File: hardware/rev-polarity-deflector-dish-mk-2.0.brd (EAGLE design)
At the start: 22.9 x 17.8 mm, 13 parts, among them U1_ ROTARY_ENCODER_SWITCH, U2 Tiny85

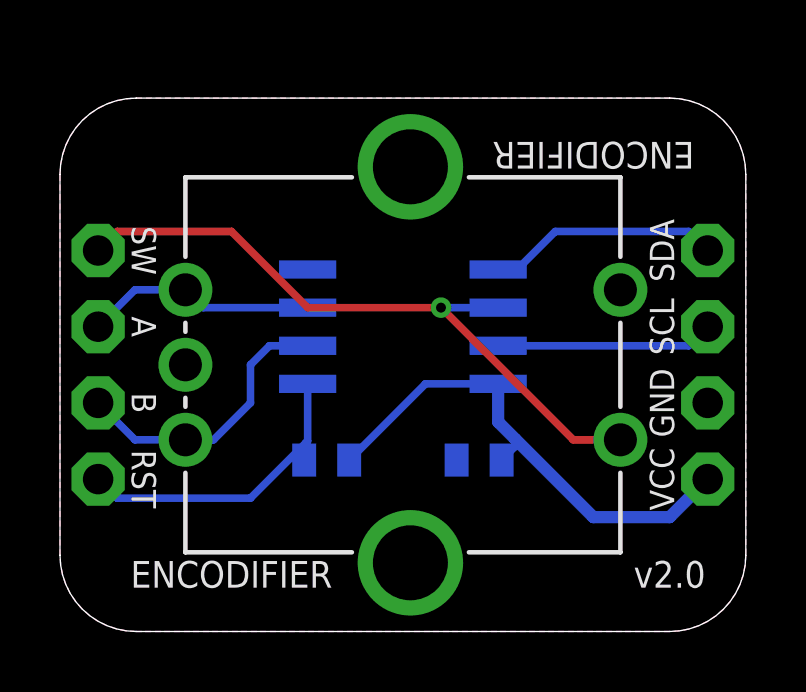
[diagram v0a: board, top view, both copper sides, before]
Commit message: have some boards, dawg
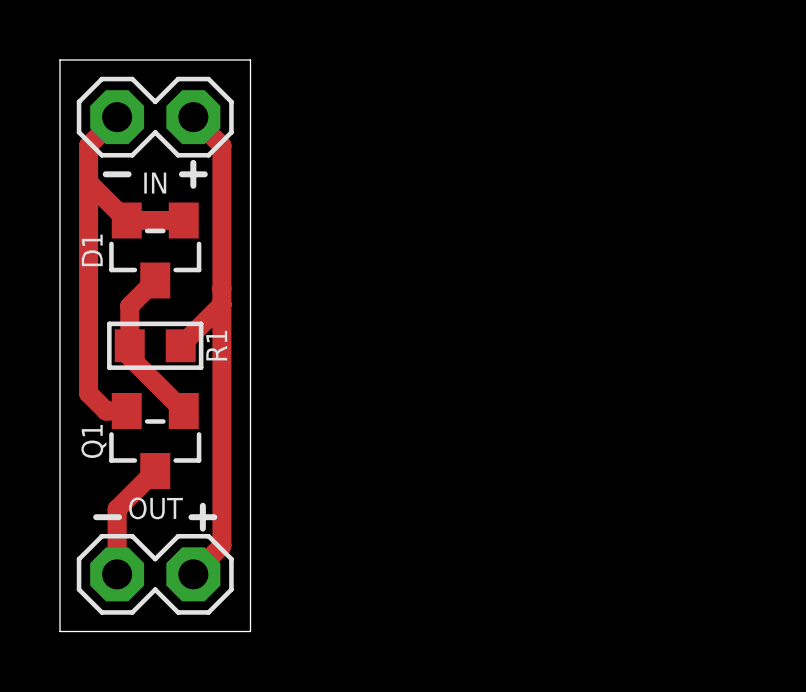
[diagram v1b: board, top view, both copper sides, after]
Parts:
- removed A, B, GND, RST, SCL, SDA, SW, VCC: M01PTH-1MM, a_parts:1X01-1MM-NS
- removed C1: 100n, a_parts:C0603-TIGHTER
- removed U1_: ROTARY_ENCODER_SWITCH, a_parts:ROTARY_ENCODER_SWITCH
- removed U2: Tiny85, a_parts:SO08-EIAJ
- added D1: 1N4740, a_parts:SOT23
- added IN, OUT: M02PTH-CENTERED, a_parts:1X02-CENTER
- added Q1: 2N7000, a_parts:SOT23
- R1: value 10k -> 100K; device a_parts:R0603-TIGHTER -> a_parts:R0603
- moved R1 6.87 mm to (3.17, 9.53), flipped to the top
- moved FRAME1 0.90 mm to (0.64, 0.64)
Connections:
- removed net A: A.1, U1_.A, U2.3
- removed net B: B.1, U1_.B, U2.2
- removed net GND: C1.2, GND.1, U1_.C, U1_.SW2, U2.4
- removed net MOSI/SDA: SDA.1, U2.5
- removed net RST: R1.1, RST.1, U2.1
- removed net SCK/SCL: SCL.1, U2.7
- removed net SW: SW.1, U1_.SW1, U2.6
- new net N$1: D1.3, Q1.1, R1.2
- new net VIN-: D1.1, D1.2, IN.1, Q1.2
- new net VOUT-: OUT.1, Q1.3
- net VCC: now also IN.2, OUT.2, R1.1; no longer C1.1, R1.2, U2.8, VCC.1
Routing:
- net SW: track 22.5 -> 0.00 mm, vias 1 -> 0
- net VIN-: track 0.00 -> 14.8 mm
- net RST: track 10.5 -> 0.00 mm
- net B: track 9.54 -> 0.00 mm
- net MOSI/SDA: track 7.77 -> 0.00 mm
- net A: track 7.74 -> 0.00 mm
- net SCK/SCL: track 7.25 -> 0.00 mm
- net N$1: track 0.00 -> 5.45 mm
- net VOUT-: track 0.00 -> 3.97 mm
- net VCC: track 17.0 -> 18.0 mm
- removed copper zone on layer 1, net GND
- removed copper zone on layer 16, net GND
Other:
- board size 22.9 x 17.8 mm -> 6.3 x 19.1 mm
- board text removed: ">VERSION"
- board text removed: "A"
- board text removed: "B"
- board text removed: "C"
- board text removed: "COM"
- board text removed: "ENCODIFIER"
- board text removed: "SW"
